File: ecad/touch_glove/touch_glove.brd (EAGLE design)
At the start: 70.4 x 40.6 mm, 184 parts, among them Q1 MCH3474 4A/30V, Q2 MCH3474 4A/30V, Q3 MCH3474 4A/30V, Q4 MCH3474 4A/30V, Q5 MCH3474 4A/30V, Q6 MCH3474 4A/30V, SW1 4A/28V, Y2 16 MHz

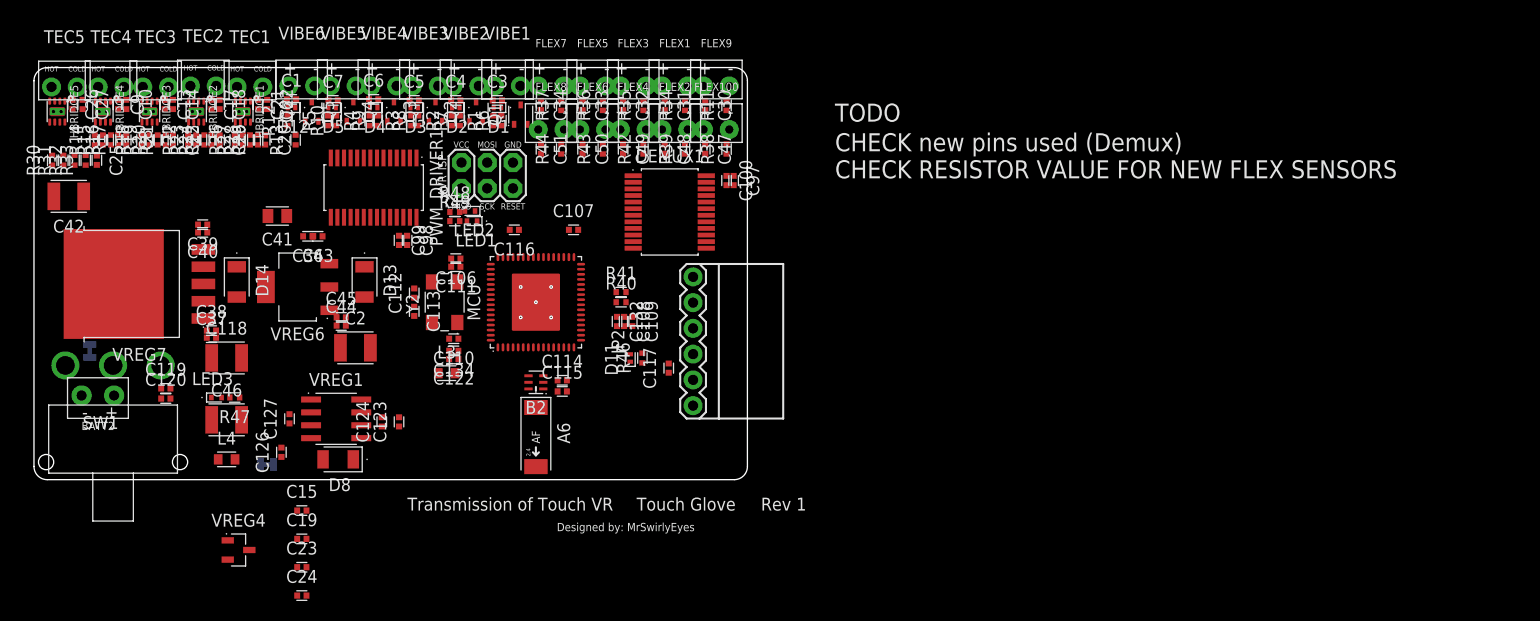
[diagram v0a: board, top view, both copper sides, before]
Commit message: Start and complete much of the 4 layer routing.  All components on board have 3D models.
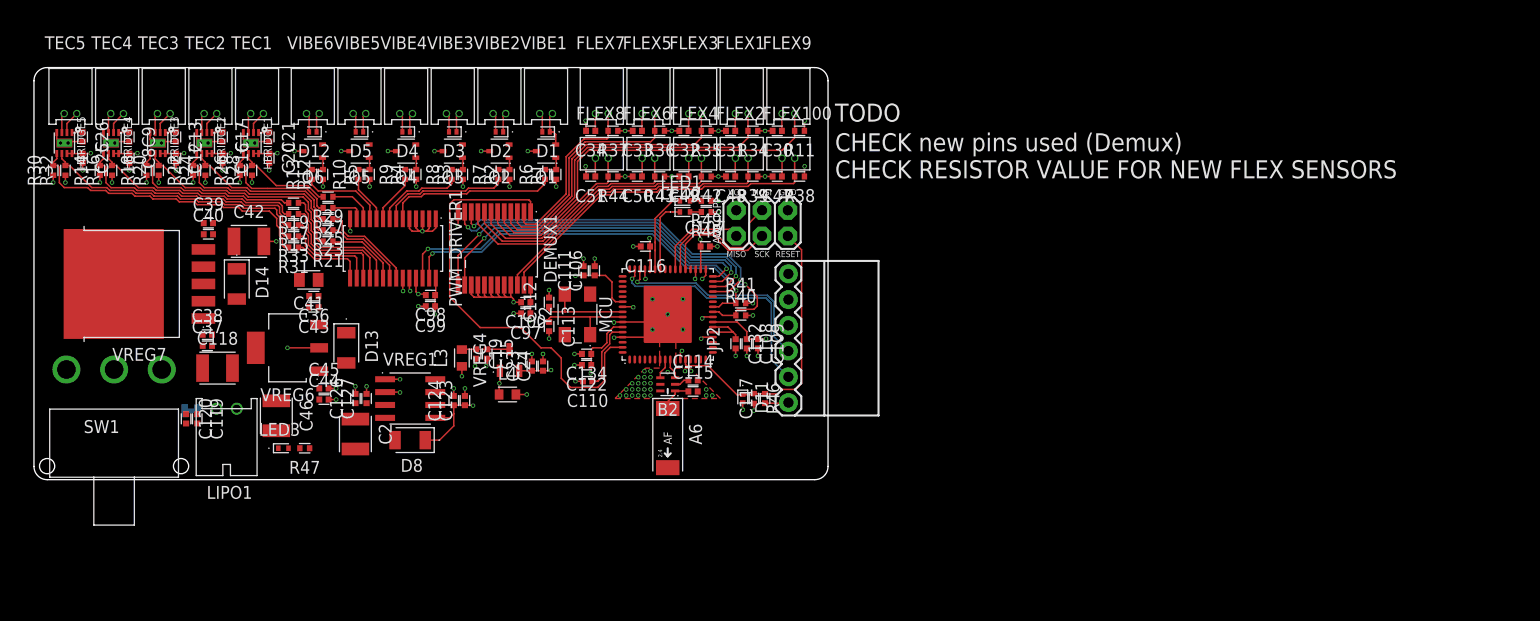
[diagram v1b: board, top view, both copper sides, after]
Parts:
- removed ANALOG_BR: 2PT_GND_TIE, PiB_power_symbols:2PT_GND_TIE
- removed BATT2: BATTERYPTH_HOLES, PiB:DUAL_PTH_PADS
- removed C1, C3, C4, C5, C6, C7: 0.1uF/50V, PiB_capacitors:CAPC1005X55_SMD-0402
- removed C10, C14, C18, C22, C27: 10uF/6.3V, PiB_capacitors:CAPC1005X55_SMD-0402
- added LIPO1: Molex RA 2mm pitch, PiB_batteries:BATTERY_MOLEX-89401_RA_PITCH-2MM
- added U$1: (no value), PiB_logo:MRSWIRLYEYES-LOGO
- AVR_ISP: value AVR ISP -> AVRISP
- FLEX1, FLEX3, FLEX5, FLEX7, FLEX9: device PiB:CONNECTOR_FSR -> PiB_sensors:_MOLEX-0530480210_RA_PITCH-1.25MM
- FLEX100, FLEX2, FLEX4, FLEX6, FLEX8: device PiB:CONNECTOR_FSR -> PiB_sensors:_MOLEX-0530470210_VERT_PITCH-1.25MM
- HBRIDGE1, HBRIDGE2, HBRIDGE3, HBRIDGE4, HBRIDGE5: value DRV8837C -> DRV8837C 1A
- JP2: value (none) -> FTDI
- TEC1, TEC2, TEC3, TEC4, TEC5: value PELTIER -> Molex RA 1.25mm pitch; device PiB:CONNECTOR_PELTIER -> PiB_actuators:_MOLEX-0530480210_RA_PITCH-1.25MM
- VIBE1, VIBE2, VIBE3, VIBE4, VIBE5, VIBE6: value VIBE_MOTOR -> Molex RA 1.25mm pitch; device PiB:CONNECTOR_VIBE-MOTOR -> PiB_actuators:_MOLEX-0530480210_RA_PITCH-1.25MM
- moved C24 32.8 mm to (50.2, 11.2), turned to 90 degrees
- moved VREG4 32.6 mm to (46.9, 11.8), turned to 90 degrees
- moved C23 30.1 mm to (49.1, 11.2), turned to 90 degrees
- moved L4 28.4 mm to (46.7, 8.40)
- moved AVR_ISP 27.5 mm to (71.8, 25.3)
- moved C19 25.1 mm to (43.6, 12.4), turned to 270 degrees
- moved R49 24.9 mm to (66.3, 27.5), turned to 180 degrees
- moved R48 24.8 mm to (66.3, 26.4), turned to 180 degrees
- moved C97 24.3 mm to (48.5, 16.4), turned to 180 degrees
- moved R31 24.3 mm to (25.6, 22.9), turned to 180 degrees
- moved C15 23.9 mm to (44.7, 12.4), turned to 270 degrees
- moved C100 23.2 mm to (48.5, 17.5), turned to 180 degrees
- moved R33 21.8 mm to (25.6, 24.0), turned to 180 degrees
- moved LED2 21.2 mm to (64.2, 26.4), turned to 0 degrees
- moved LED1 21.1 mm to (64.2, 27.5), turned to 0 degrees
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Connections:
- removed net BATT_+: BATT2.+, SW1.S1
- removed net C10: DEMUX1.21
- removed net C11: DEMUX1.20
- removed net C12: DEMUX1.19
- removed net C13: DEMUX1.18
- removed net C8: DEMUX1.23
- removed net C9: DEMUX1.22
- removed net N$52: ANALOG_BR.P$1, L4.2
- new net +: LIPO1.+, SW1.S1
- net 1.8V: no longer C10.1, C14.1, C18.1, C22.1, C27.1
- net 3.3V: no longer C1.1, C3.1, C4.1, C5.1, C6.1, C7.1
- net A0: now also DEMUX1.1
- net A1: no longer DEMUX1.1
- net AGND: now also B2.5, C110.2, C114.2, C115.2, DEMUX1.16, DEMUX1.17, DEMUX1.18, DEMUX1.19, DEMUX1.20, DEMUX1.21, L4.2, MCU.10, MCU.7, MCU.P$1, MCU.P$2, MCU.P$3, MCU.P$4, MCU.P$5; no longer ANALOG_BR.P$2
- net AVCC: now also FLEX1.1, FLEX100.1, FLEX2.1, FLEX3.1, FLEX4.1, FLEX5.1, FLEX6.1, FLEX7.1, FLEX8.1, FLEX9.1; no longer FLEX1.+, FLEX100.+, FLEX2.+, FLEX3.+, FLEX4.+, FLEX5.+, FLEX6.+, FLEX7.+, FLEX8.+, FLEX9.+
- net GND: now also AVR_ISP.GND, LIPO1.-, R1.1, R12.1, R2.1, R3.1, R4.1, R5.1; no longer AVR_ISP.6, B2.5, BATT2.-, C110.2, C114.2, C115.2, MCU.10, MCU.7
- net MISO: now also AVR_ISP.MISO; no longer AVR_ISP.1
- net MOSI: now also AVR_ISP.MOSI; no longer AVR_ISP.4
- net N$1: now also TEC5.1; no longer TEC5.HOT
- net N$11: now also TEC4.1; no longer TEC4.HOT
- net N$12: now also TEC3.1; no longer TEC3.HOT
- net N$15: no longer C4.2
- net N$16: now also TEC3.2; no longer TEC3.COLD
- net N$17: no longer C3.2
- net N$18: now also TEC2.1; no longer TEC2.HOT
- net N$2: no longer C6.2
- net N$23: now also TEC2.2; no longer TEC2.COLD
- net N$24: now also TEC1.1; no longer TEC1.HOT
- net N$27: now also TEC1.2; no longer TEC1.COLD
- net N$3: no longer C7.2
- net N$30: no longer C1.2
- net N$4: no longer C5.2
- net N$5: now also TEC5.2; no longer TEC5.COLD
- net N$6: now also TEC4.2; no longer TEC4.COLD
- net NGND: now also VREG7.6; no longer C10.2, C14.2, C18.2, C22.2, C27.2, R1.1, R12.1, R2.1, R3.1, R4.1, R5.1
- net PD4: now also DEMUX1.10; no longer DEMUX1.13
- net PD5: now also DEMUX1.11; no longer DEMUX1.14
- net PD6: now also DEMUX1.13; no longer DEMUX1.11
- net PD7: now also DEMUX1.14; no longer DEMUX1.10
- net RESET: now also AVR_ISP.RESET; no longer AVR_ISP.5
- net SCK: now also AVR_ISP.SCK; no longer AVR_ISP.3
- net STRAIN_1: now also DEMUX1.5, FLEX1.2; no longer DEMUX1.9, FLEX1.-
- net STRAIN_10: now also DEMUX1.23, FLEX100.2; no longer DEMUX1.16, FLEX100.-
- net STRAIN_2: now also DEMUX1.22, FLEX2.2; no longer DEMUX1.8, FLEX2.-
- net STRAIN_3: now also DEMUX1.4, FLEX3.2; no longer DEMUX1.7, FLEX3.-
- net STRAIN_4: now also DEMUX1.9, FLEX4.2; no longer DEMUX1.6, FLEX4.-
- net STRAIN_5: now also DEMUX1.3, FLEX5.2; no longer DEMUX1.5, FLEX5.-
- net STRAIN_6: now also DEMUX1.8, FLEX6.2; no longer DEMUX1.4, FLEX6.-
- net STRAIN_7: now also DEMUX1.2, FLEX7.2; no longer DEMUX1.3, FLEX7.-
- net STRAIN_8: now also DEMUX1.7, FLEX8.2; no longer DEMUX1.2, FLEX8.-
- net STRAIN_9: now also DEMUX1.6, FLEX9.2; no longer DEMUX1.17, FLEX9.-
- net TEC_1_COLD: now also PWM_DRIVER1.13; no longer PWM_DRIVER1.12
- net TEC_1_HOT: now also PWM_DRIVER1.12; no longer PWM_DRIVER1.13
- net VCC: no longer AVR_ISP.2, JP2.VCC
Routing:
- net GND: track 0.00 -> 57.7 mm, vias 0 -> 56
- net VCC: track 0.00 -> 49.6 mm, vias 0 -> 16
- net AGND: track 0.00 -> 48.8 mm, vias 0 -> 49
- net SCL: track 0.00 -> 45.1 mm, vias 0 -> 2
- net A0: track 0.00 -> 43.6 mm
- net STRAIN_9: track 0.00 -> 39.4 mm
- net SDA: track 0.00 -> 39.4 mm, vias 0 -> 2
- net PD6: track 0.00 -> 35.5 mm, vias 0 -> 2
- net PD4: track 0.00 -> 34.5 mm, vias 0 -> 2
- net STRAIN_10: track 0.00 -> 34.0 mm
- net PD5: track 0.00 -> 33.9 mm, vias 0 -> 2
- net STRAIN_1: track 0.00 -> 33.9 mm
- net PD7: track 0.00 -> 33.1 mm, vias 0 -> 2
- net AVCC: track 0.00 -> 31.2 mm, vias 0 -> 3
- net N$29: track 0.00 -> 30.0 mm
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- added copper zone on layer 1, net AGND
- added copper zone on layer 15, net AGND
- added copper zone on layer 2, net AGND
- added copper zone on layer 2, net AVCC
- added copper zone on layer 15, net N$34
- added copper zone on layer 2, net N$34
- added copper zone on layer 15, net NGND
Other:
- board size 70.4 x 40.6 mm -> 78.3 x 40.6 mm
- board text added: "Touch Glove Rev 2"
- board text removed: "Touch Glove Rev 1"
